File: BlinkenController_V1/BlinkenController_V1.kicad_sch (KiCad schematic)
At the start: 44 parts, among them J1 Conn_01x02_Socket, J2 Conn_01x08_Socket, J4 Conn_01x03_Socket, J5 6P6C, J6 6P6C, J7 Conn_01x04_Pin, J8 Conn_01x06_Socket, SW1 SW_DIP_x01, SW2 SW_Push, SW3 SW_Push, SW4 SW_Push, SW5 SW_Push, SW6 SW_Push, U1 Pico, U2 MAX232, U3 TL331, U4 MAX3485

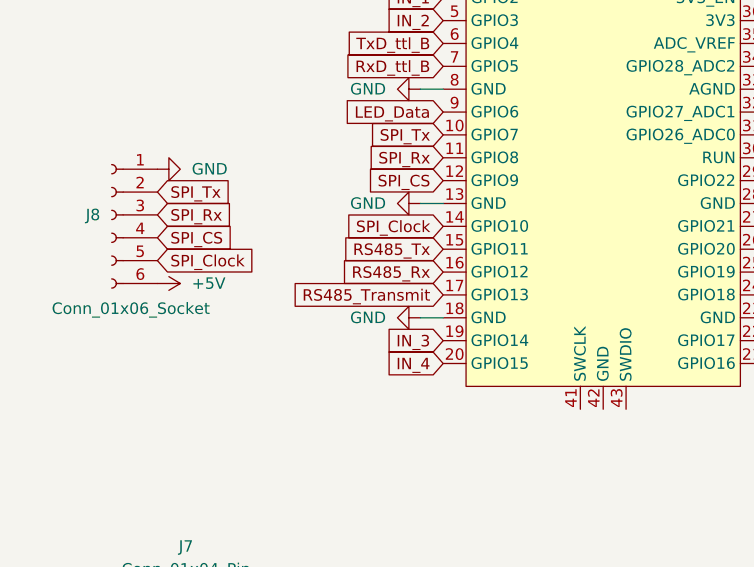
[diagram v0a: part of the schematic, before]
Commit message: Improved board density
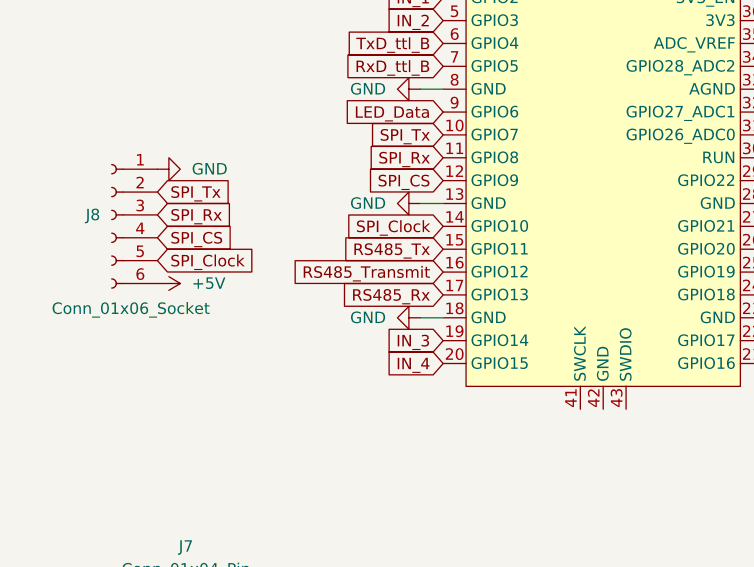
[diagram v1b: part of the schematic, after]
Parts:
- C2: footprint Capacitor_THT:C_Radial_D6.3mm_H7.0mm_P2.50mm -> Capacitor_THT:C_Disc_D5.0mm_W2.5mm_P5.00mm
- C3: footprint Capacitor_THT:C_Radial_D6.3mm_H5.0mm_P2.50mm -> Capacitor_THT:C_Disc_D5.0mm_W2.5mm_P5.00mm
- J1: footprint Connector_Wago:Wago_734-132_1x02_P3.50mm_Vertical -> Connector_Phoenix_MSTB:PhoenixContact_MSTBVA_2,5_2-G_1x02_P5.00mm_Vertical
- J4: footprint Connector_Wago:Wago_734-133_1x03_P3.50mm_Vertical -> Connector_Phoenix_MSTB:PhoenixContact_MSTBVA_2,5_3-G_1x03_P5.00mm_Vertical
- J7: footprint Connector_Wago:Wago_734-134_1x04_P3.50mm_Vertical -> Connector_Phoenix_MSTB:PhoenixContact_MSTBVA_2,5_4-G_1x04_P5.00mm_Vertical
- SW2, SW3, SW4, SW5, SW6: footprint Button_Switch_SMD:SW_SPST_PTS810 -> Button_Switch_SMD:SW_Tactile_SPST_NO_Straight_CK_PTS636Sx25SMTRLFS
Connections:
- net RS485_Rx: now also U1.17 (GPIO13); no longer U1.16 (GPIO12)
- net RS485_Transmit: now also U1.16 (GPIO12); no longer U1.17 (GPIO13)
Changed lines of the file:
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@@
 	(global_label "RS485_Transmit"
 		(shape input)
-		(at 58.42 68.58 180)
+		(at 58.42 66.04 180)
 		(fields_autoplaced yes)
 		(effects
@@
 		)
 		(property "Intersheetrefs" "${INTERSHEET_REFS}"
-			(at 40.2555 68.58 0)
+			(at 40.2555 66.04 0)
 			(effects
 				(font
@@
 	(global_label "RS485_Rx"
 		(shape input)
-		(at 58.42 66.04 180)
+		(at 58.42 68.58 180)
 		(fields_autoplaced yes)
 		(effects
@@
 		)
 		(property "Intersheetrefs" "${INTERSHEET_REFS}"
-			(at 46.0611 66.04 0)
+			(at 46.0611 68.58 0)
 			(effects
 				(font
@@
 			)
 		)
-		(property "Footprint" "Button_Switch_SMD:SW_SPST_PTS810"
+		(property "Footprint" "Button_Switch_SMD:SW_Tactile_SPST_NO_Straight_CK_PTS636Sx25SMTRLFS"
 			(at 139.7 143.51 0)
 			(effects
@@
 			)
 		)
-		(property "Footprint" "Button_Switch_SMD:SW_SPST_PTS810"
+		(property "Footprint" "Button_Switch_SMD:SW_Tactile_SPST_NO_Straight_CK_PTS636Sx25SMTRLFS"
 			(at 50.8 143.51 0)
 			(effects
@@
 			)
 		)
-		(property "Footprint" "Connector_Wago:Wago_734-133_1x03_P3.50mm_Vertical"
+		(property "Footprint" "Connector_Phoenix_MSTB:PhoenixContact_MSTBVA_2,5_3-G_1x03_P5.00mm_Vertical"
 			(at 260.35 86.36 0)
 			(effects
@@
 			)
 		)
-		(property "Footprint" "Button_Switch_SMD:SW_SPST_PTS810"
+		(property "Footprint" "Button_Switch_SMD:SW_Tactile_SPST_NO_Straight_CK_PTS636Sx25SMTRLFS"
 			(at 80.01 143.51 0)
 			(effects
@@
 			)
 		)
-		(property "Footprint" "Capacitor_THT:C_Radial_D6.3mm_H7.0mm_P2.50mm"
+		(property "Footprint" "Capacitor_THT:C_Disc_D5.0mm_W2.5mm_P5.00mm"
 			(at 225.7552 46.99 0)
 			(effects
@@
 			)
 		)
-		(property "Footprint" "Connector_Wago:Wago_734-132_1x02_P3.50mm_Vertical"
+		(property "Footprint" "Connector_Phoenix_MSTB:PhoenixContact_MSTBVA_2,5_2-G_1x02_P5.00mm_Vertical"
 			(at 35.56 154.94 0)
 			(effects
@@
 			)
 		)
-		(property "Footprint" "Capacitor_THT:C_Radial_D6.3mm_H5.0mm_P2.50mm"
+		(property "Footprint" "Capacitor_THT:C_Disc_D5.0mm_W2.5mm_P5.00mm"
 			(at 177.4952 46.99 0)
 			(effects
@@
 			)
 		)
-		(property "Footprint" "Button_Switch_SMD:SW_SPST_PTS810"
+		(property "Footprint" "Button_Switch_SMD:SW_Tactile_SPST_NO_Straight_CK_PTS636Sx25SMTRLFS"
 			(at 109.22 143.51 0)
 			(effects
@@
 			)
 		)
-		(property "Footprint" "Connector_Wago:Wago_734-134_1x04_P3.50mm_Vertical"
+		(property "Footprint" "Connector_Phoenix_MSTB:PhoenixContact_MSTBVA_2,5_4-G_1x04_P5.00mm_Vertical"
 			(at 29.21 104.14 0)
 			(effects
@@
 			)
 		)
-		(property "Footprint" "Button_Switch_SMD:SW_SPST_PTS810"
+		(property "Footprint" "Button_Switch_SMD:SW_Tactile_SPST_NO_Straight_CK_PTS636Sx25SMTRLFS"
 			(at 137.16 44.45 0)
 			(effects
